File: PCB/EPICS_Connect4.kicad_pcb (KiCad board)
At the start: 2 copper layers, 50 x 50 mm, 57 parts, among them J1 USB_C_Receptacle_USB2.0_14P, J2 TC2030, J3 Power, J4 EndA, J5 EndB, J6 LEDA, J7 LEDB, J8 Motor, SW1 ESP.RST, SW2 ESP.BOOT, U2 TPS54202DDC, U3 AP2205-5, U4 SN74AHCT1G125DBVR, U5 ESP32-C3-WROOM-02, U6 SN74AHCT1G125DBVR, U7 STM32G474CBTx

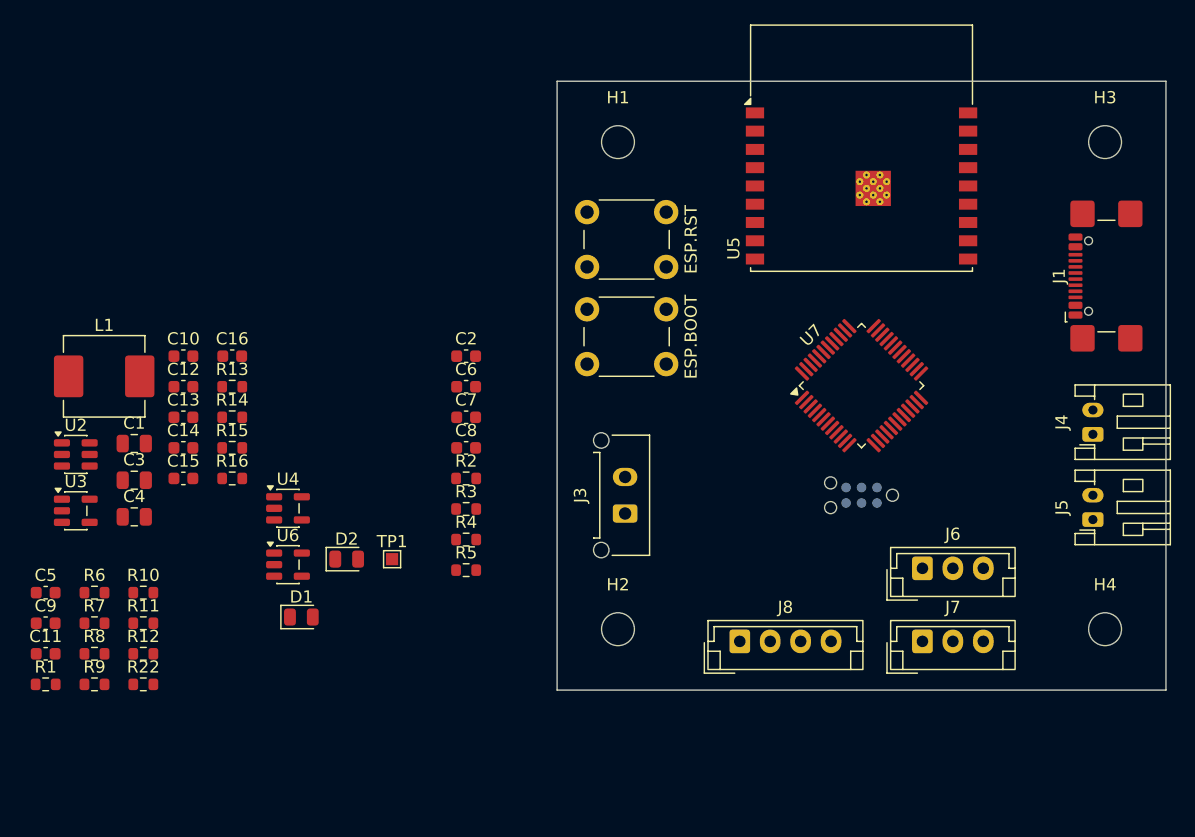
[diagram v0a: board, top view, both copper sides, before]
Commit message: Update EPICS_Connect4 KiCad project
Co-Authored-By: Claude Sonnet 5 <noreply@anthropic.com>
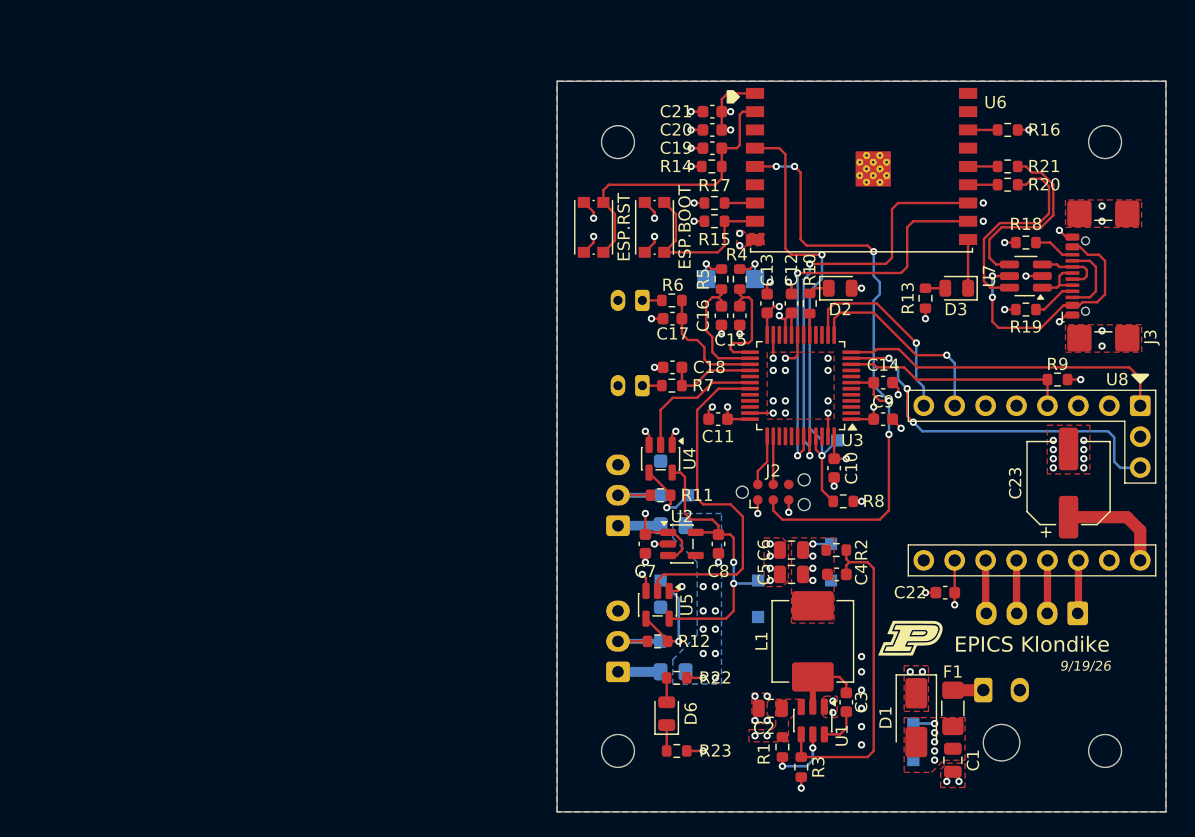
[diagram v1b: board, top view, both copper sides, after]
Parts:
- added C17: 0.1uF, Capacitor_SMD:C_0603_1608Metric, F.Cu at (134.5, 94.5)
- added C18: 0.1uF, Capacitor_SMD:C_0603_1608Metric, F.Cu at (134.5, 98.5)
- added C19: 1uF, Capacitor_SMD:C_0603_1608Metric, F.Cu at (137.8, 80.5)
- added C20: 10uF, Capacitor_SMD:C_0603_1608Metric, F.Cu at (137.8, 79.0)
- added C21: 10uF, Capacitor_SMD:C_0603_1608Metric, F.Cu at (137.8, 77.5)
- added C22: 1uF, Capacitor_SMD:C_0603_1608Metric, F.Cu at (156.9, 117.0)
- added C23: 100uF, Capacitor_SMD:CP_Elec_6.3x5.9, F.Cu at (167.0, 108.0)
- added D3: 4.5mA @ 1.8V, LED_SMD:LED_0805_2012Metric, F.Cu at (157.8, 92.0)
- added D4: SMF5.0A, Diode_SMD:D_SOD-123F, B.Cu at (133.5, 107.6)
- added D5: SMF5.0A, Diode_SMD:D_SOD-123F, B.Cu at (133.5, 119.6)
- added D6: LED_Small, LED_SMD:LED_0805_2012Metric, F.Cu at (134.0, 126.9)
- added F1: 5A, Fuse:Fuse_1206_3216Metric_Pad1.42x1.75mm_HandSolder, F.Cu at (157.5, 126.5)
- added F2: 2A, Fuse:Fuse_0805_2012Metric_Pad1.15x1.40mm_HandSolder, B.Cu at (134.5, 111.5)
- added F3: 2A, Fuse:Fuse_0805_2012Metric_Pad1.15x1.40mm_HandSolder, B.Cu at (134.5, 123.5)
- added R17: 10k, Resistor_SMD:R_0603_1608Metric, F.Cu at (137.9, 85.0)
- added R18: 5.1k, Resistor_SMD:R_0603_1608Metric, F.Cu at (163.5, 88.2)
- added R19: 5.1k, Resistor_SMD:R_0603_1608Metric, F.Cu at (163.5, 93.8)
- added R20: 22, Resistor_SMD:R_0603_1608Metric, F.Cu at (162.0, 83.5)
- added R21: 22, Resistor_SMD:R_0603_1608Metric, F.Cu at (162.0, 82.0)
- added R23: 330, Resistor_SMD:R_0603_1608Metric, F.Cu at (134.8, 130.0)
- added SYM1: Logo_Open_Hardware_Large, Library:S_Silk_Logo, F.Cu at (154.0, 120.8)
- added TP10: INRP.A, TestPoint:TestPoint_Pad_1.5x1.5mm, B.Cu at (141.2, 91.2)
- added TP11: INRP.B, TestPoint:TestPoint_Pad_1.5x1.5mm, B.Cu at (137.2, 91.2)
- added TP2: GND, TestPoint:TestPoint_Pad_1.0x1.0mm, B.Cu at (154.2, 130.8)
- added TP3: +5V, TestPoint:TestPoint_Pad_1.0x1.0mm, B.Cu at (141.5, 116.0)
- added TP4: GND, TestPoint:TestPoint_Pad_1.0x1.0mm, B.Cu at (141.5, 119.0)
- added TP5: +3V3, TestPoint:TestPoint_Pad_1.0x1.0mm, B.Cu at (147.5, 113.0)
- added TP6: GND, TestPoint:TestPoint_Pad_1.0x1.0mm, B.Cu at (147.5, 116.0)
- added TP7: ST.BOOT, TestPoint:TestPoint_Pad_1.0x1.0mm, B.Cu at (148.0, 104.5)
- added TP8: DataA, TestPoint:TestPoint_Pad_1.0x1.0mm, B.Cu at (135.8, 109.0)
- added TP9: DataB, TestPoint:TestPoint_Pad_1.0x1.0mm, B.Cu at (133.5, 116.0)
- added U1: TPS54202DDC, Package_TO_SOT_SMD:SOT-23-6, F.Cu at (146.0, 127.5)
- added U8: TMC2209, Library:STEPSTICK_socket, F.Cu at (164.0, 108.0)
- C11, C7, C9: value 10uF -> 1uF
- C14, C15: value 1uF -> 0.1uF
- C2: value 0.1uF -> 10uF; footprint Capacitor_SMD:C_0603_1608Metric -> Capacitor_SMD:C_0805_2012Metric
- C3: value 22uF -> 0.1uF; footprint Capacitor_SMD:C_0805_2012Metric -> Capacitor_SMD:C_0603_1608Metric
- C4: value 22uF -> 56pF; footprint Capacitor_SMD:C_0805_2012Metric -> Capacitor_SMD:C_0603_1608Metric
- C5, C6: value 1uF -> 22uF; footprint Capacitor_SMD:C_0603_1608Metric -> Capacitor_SMD:C_0805_2012Metric
- C8: value 56pF -> 10uF
- D1: value 4.5mA @ 1.8V -> SMAJ12A; footprint LED_SMD:LED_0805_2012Metric -> Diode_SMD:D_SMA
- J1: value USB_C_Receptacle_USB2.0_14P -> Power; footprint Connector_USB:USB_C_Receptacle_GCT_USB4110 -> Connector_Molex:Molex_Micro-Fit_3.0_43650-0200_1x02_P3.00mm_Horizontal; moved to B.Cu
- J2: moved to F.Cu
- J3: value Power -> USB_C_Receptacle_USB2.0_14P; footprint Connector_Molex:Molex_Micro-Fit_3.0_43650-0215_1x02_P3.00mm_Vertical -> Connector_USB:USB_C_Receptacle_GCT_USB4110
- J4, J5: footprint Connector_JST:JST_PH_S2B-PH-K_1x02_P2.00mm_Horizontal -> Connector_JST:JST_PH_B2B-PH-K_1x02_P2.00mm_Vertical; moved to B.Cu
- J6, J7, J8: moved to B.Cu
- R1: value 5.1k -> 510k
- R10, R7: value 10k -> 330
- R11, R22: value 5.1k -> 330
- R12: value 22 -> 330
- R13: value 75 -> 330
- R14: value 75 -> 10k
- R15: value 330 -> 10k
- R2: value 22.1k -> 100k
- R3: value 330k -> 22.1k
- R4: value 100k -> 330
- R5: value 56k -> 330
- R9: value 10k -> 5.1k
- SW1, SW2: footprint Button_Switch_THT:SW_PUSH_6mm_H4.3mm -> Button_Switch_SMD:SW_Push_1P1T_NO_CK_KMR2
- TP1: value ST.BOOT -> +12V; moved to B.Cu
- U2: value TPS54202DDC -> AP2205-5; footprint Package_TO_SOT_SMD:SOT-23-6 -> Package_TO_SOT_SMD:SOT-23-5
- U3: value AP2205-5 -> STM32G474CBTx; footprint Package_TO_SOT_SMD:SOT-23-5 -> Package_QFP:LQFP-48_7x7mm_P0.5mm
- U5: value ESP32-C3-WROOM-02 -> SN74AHCT1G125DBVR; footprint RF_Module:ESP32-C3-WROOM-02 -> Package_TO_SOT_SMD:SOT-23-5
- U6: value SN74AHCT1G125DBVR -> ESP32-C3-WROOM-02; footprint Package_TO_SOT_SMD:SOT-23-5 -> RF_Module:ESP32-C3-WROOM-02
- U7: value STM32G474CBTx -> USBLC6-2SC6; footprint Package_QFP:LQFP-48_7x7mm_P0.5mm -> Package_TO_SOT_SMD:SOT-23-6_Handsoldering
- moved R9 83.0 mm to (166.1, 99.5), turned to 180 degrees
- moved C1 72.1 mm to (157.5, 130.8), turned to -90 degrees
- moved C9 70.8 mm to (151.8, 102.8)
- moved R16 69.8 mm to (162.0, 79.0), turned to 180 degrees
- moved R8 62.8 mm to (148.5, 109.5)
- moved L1 62.1 mm to (146.0, 121.0), turned to 90 degrees
- moved C5 61.3 mm to (144.2, 115.5)
- moved C3 61.3 mm to (148.8, 126.0), turned to 90 degrees
- moved R1 60.7 mm to (143.5, 129.7), turned to -90 degrees
- moved U3 60.4 mm to (145.0, 100.0), turned to 180 degrees
- moved R10 59.7 mm to (145.8, 93.2), turned to -90 degrees
- moved C11 58.5 mm to (138.2, 102.8), turned to 180 degrees
- moved C4 57.9 mm to (148.0, 115.5), turned to 180 degrees
- moved C14 57.7 mm to (151.8, 99.8)
- moved R13 57.4 mm to (155.2, 92.8), turned to 90 degrees
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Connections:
- C1 pad 1: GND -> +12V
- C1 pad 2: /Power Regulators/VIN -> GND
- C14 pad 1: +3V3 -> /STM32 Controller/NRST
- C15 pad 1: +3V3 -> /STM32 Controller/INRP.A*
- C16 pad 1: /STM32 Controller/NRST -> /STM32 Controller/INRP.B*
- C2 pad 1: Net-(U2-BOOT) -> GND
- C2 pad 2: Net-(U2-SW) -> +12V
- C3 pad 1: GND -> Net-(U1-BOOT)
- C3 pad 2: /Power Regulators/+3V3 -> Net-(U1-SW)
- C4 pad 1: GND -> Net-(U1-FB)
- C4 pad 2: /Power Regulators/+3V3 -> +3V3
- C5 pad 1: /ESP32 Weblink/EN -> GND
- C5 pad 2: GND -> +3V3
- C6 pad 2: /Power Regulators/VIN -> +3V3
- C7 pad 2: /Power Regulators/+5V -> +12V
- C8 pad 1: Net-(U2-FB) -> GND
- C8 pad 2: /Power Regulators/+3V3 -> +5V
- D1 pad 1: /ESP32 Weblink/LED -> GND
- D1 pad 2: Net-(D1-A) -> +12V
- D2 pad 1: /STM32 Controller/U_LED -> Net-(D2-K)
- D2 pad 2: Net-(D2-A) -> +3V3
- J4 pad 1: unconnected-(J4-Pin_1-Pad1) -> /STM32 Controller/END.A
- J4 pad 2: unconnected-(J4-Pin_2-Pad2) -> GND
- J5 pad 1: unconnected-(J5-Pin_1-Pad1) -> /STM32 Controller/END.B
- J5 pad 2: unconnected-(J5-Pin_2-Pad2) -> GND
- J6 pad 1: unconnected-(J6-Pin_1-Pad1) -> Net-(J6-Pin_1)
- J6 pad 2: unconnected-(J6-Pin_2-Pad2) -> /STM32 Controller/ledDataA
- J6 pad 3: unconnected-(J6-Pin_3-Pad3) -> GND
- J7 pad 1: unconnected-(J7-Pin_1-Pad1) -> Net-(J7-Pin_1)
- J7 pad 2: unconnected-(J7-Pin_2-Pad2) -> /STM32 Controller/ledDataB
- J7 pad 3: unconnected-(J7-Pin_3-Pad3) -> GND
- J8 pad 1: unconnected-(J8-Pin_1-Pad1) -> /Motor Acuator/M10
- J8 pad 2: unconnected-(J8-Pin_2-Pad2) -> /Motor Acuator/M11
- J8 pad 3: unconnected-(J8-Pin_3-Pad3) -> /Motor Acuator/M12
- J8 pad 4: unconnected-(J8-Pin_4-Pad4) -> /Motor Acuator/M13
- L1 pad 1: Net-(U2-SW) -> Net-(U1-SW)
- L1 pad 2: /Power Regulators/+3V3 -> +3V3
- R1 pad 1: Net-(J1-CC1) -> +12V
- R1 pad 2: GND -> Net-(U1-EN)
- R10 pad 1: +3V3 -> Net-(D2-K)
- R10 pad 2: /ESP32 Weblink/IO8 -> /STM32 Controller/U_LED
- R11 pad 1: Net-(J1-CC2) -> Net-(U4-Y)
- R11 pad 2: GND -> /STM32 Controller/ledDataA
- R12 pad 1: Net-(J1-D--PadA7) -> Net-(U5-Y)
- R12 pad 2: /ESP32 Weblink/D- -> /STM32 Controller/ledDataB
- R13 pad 1: Net-(U4-Y) -> +3V3
- R13 pad 2: /STM32 Controller/ledDataA -> Net-(D3-A)
- R14 pad 1: Net-(U6-Y) -> +3V3
- R14 pad 2: /STM32 Controller/ledDataB -> /ESP32 Weblink/EN
- R15 pad 2: Net-(D2-A) -> /ESP32 Weblink/IO9
- R16 pad 1: /STM32 Controller/BOOT -> +3V3
- R16 pad 2: GND -> /ESP32 Weblink/IO2
- R2 pad 1: Net-(U2-FB) -> +3V3
- R2 pad 2: GND -> Net-(U1-FB)
- R22 pad 1: Net-(J1-D+-PadA6) -> +12V
- R22 pad 2: /ESP32 Weblink/D+ -> Net-(D6-A)
- R3 pad 1: /Power Regulators/VIN -> Net-(U1-FB)
- R3 pad 2: /Power Regulators/EN -> GND
- R4 pad 1: /Power Regulators/+3V3 -> /STM32 Controller/INRP.A
- R4 pad 2: Net-(U2-FB) -> /STM32 Controller/INRP.A*
- R5 pad 1: /Power Regulators/EN -> /STM32 Controller/INRP.B
- R5 pad 2: GND -> /STM32 Controller/INRP.B*
- R6 pad 1: +3V3 -> /STM32 Controller/END.A
- R6 pad 2: Net-(D1-A) -> /STM32 Controller/END.A*
- R7 pad 1: +3V3 -> /STM32 Controller/END.B
- R7 pad 2: /ESP32 Weblink/IO2 -> /STM32 Controller/END.B*
- R8 pad 1: +3V3 -> /STM32 Controller/BOOT
- R8 pad 2: /ESP32 Weblink/IO9 -> GND
- R9 pad 2: /ESP32 Weblink/EN -> /Motor Acuator/TMC.PDN
- TP1 pad 1: /STM32 Controller/BOOT -> +12V
- U2 pad 1: GND -> +12V
- U2 pad 2: Net-(U2-SW) -> GND
- U2 pad 3: /Power Regulators/VIN -> +12V
- U2 pad 4: Net-(U2-FB) -> unconnected-(U2-NC-Pad4)
- U2 pad 5: /Power Regulators/EN -> +5V
- U3 pad 1: /Power Regulators/VIN -> +3V3
- U3 pad 2: GND -> unconnected-(U3-PC13-Pad2)
- U3 pad 3: /Power Regulators/VIN -> unconnected-(U3-PC14-Pad3)
- U3 pad 5: /Power Regulators/+5V -> unconnected-(U3-PF0-Pad5)
- U5 pad 1: +3V3 -> GND
- U5 pad 2: /ESP32 Weblink/EN -> /STM32 Controller/LED.B
- U5 pad 3: unconnected-(U5-IO4-Pad3) -> GND
- U5 pad 4: /ESP32 Weblink/BOOT -> Net-(U5-Y)
- U5 pad 5: /ESP32 Weblink/NRST -> +5V
- U6 pad 1: GND -> +3V3
- U6 pad 2: /STM32 Controller/LED.B -> /ESP32 Weblink/EN
- U6 pad 3: GND -> unconnected-(U6-IO4-Pad3)
- U6 pad 4: Net-(U6-Y) -> /STM32 Controller/BOOT
- U6 pad 5: +5V -> /STM32 Controller/NRST
- U7 pad 1: +3V3 -> Net-(J3-D--PadA7)
- U7 pad 2: unconnected-(U7-PC13-Pad2) -> GND
- U7 pad 3: unconnected-(U7-PC14-Pad3) -> Net-(J3-D+-PadA6)
- U7 pad 4: unconnected-(U7-PC15-Pad4) -> /ESP32 Weblink/D.+
- U7 pad 5: unconnected-(U7-PF0-Pad5) -> Net-(U7-VBUS)
- U7 pad 6: unconnected-(U7-PF1-Pad6) -> /ESP32 Weblink/D.-
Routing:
- net /STM32 Controller/NRST: track 0.00 -> 53.3 mm, vias 0 -> 5
- net GND: track 0.00 -> 45.6 mm, vias 0 -> 82
- net /STM32 Controller/BOOT: track 0.00 -> 38.7 mm, vias 0 -> 2
- net +3V3: track 0.00 -> 35.4 mm, vias 0 -> 20
- net /ESP32 Weblink/IO21/TXD: track 0.00 -> 35.2 mm, vias 0 -> 2
- net /ESP32 Weblink/IO20/RXD: track 0.00 -> 34.5 mm, vias 0 -> 2
- net /Motor Acuator/TMC.DIAG: track 0.00 -> 30.5 mm, vias 0 -> 3
- net /STM32 Controller/LED.B: track 0.00 -> 29.2 mm
- net Net-(U1-FB): track 0.00 -> 27.4 mm
- net /Motor Acuator/TMC.EN: track 0.00 -> 27.1 mm
- net +5V: track 0.00 -> 25.1 mm, vias 0 -> 2
- net /ESP32 Weblink/EN: track 0.00 -> 23.9 mm
- net Net-(U7-VBUS): track 0.00 -> 21.7 mm, vias 0 -> 2
- net +12V: track 0.00 -> 19.1 mm, vias 0 -> 18
- net /Motor Acuator/TMC.PDN: track 0.00 -> 18.8 mm
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- added copper zone on B.Cu, net +12V
- added copper zone on F.Cu, net +12V
- added copper zone on In2.Cu, net +12V
- added copper zone on F.Cu, net +3V3
- added copper zone on In2.Cu, net +3V3
- added copper zone on B.Cu, net GND
- added copper zone on F.Cu, net GND
- added copper zone on In1.Cu, net GND
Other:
- board size 50 x 50 mm -> 50 x 60 mm
- copper layers 2 -> 4
- board text added: "9/19/26"
- board text added: "EPICS Klondike"
